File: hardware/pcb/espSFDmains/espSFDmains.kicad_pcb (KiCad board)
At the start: 2 copper layers, 59.1 x 88.9 mm, 22 parts, among them J1 Conn_01x06_Socket, J2 Conn_02x10_Odd_Even, J3 Mains, J4 Mains Motor, U1 WeMos_D1_mini_esp32, U2 TSR_1-2450, U3 SFH617A-1

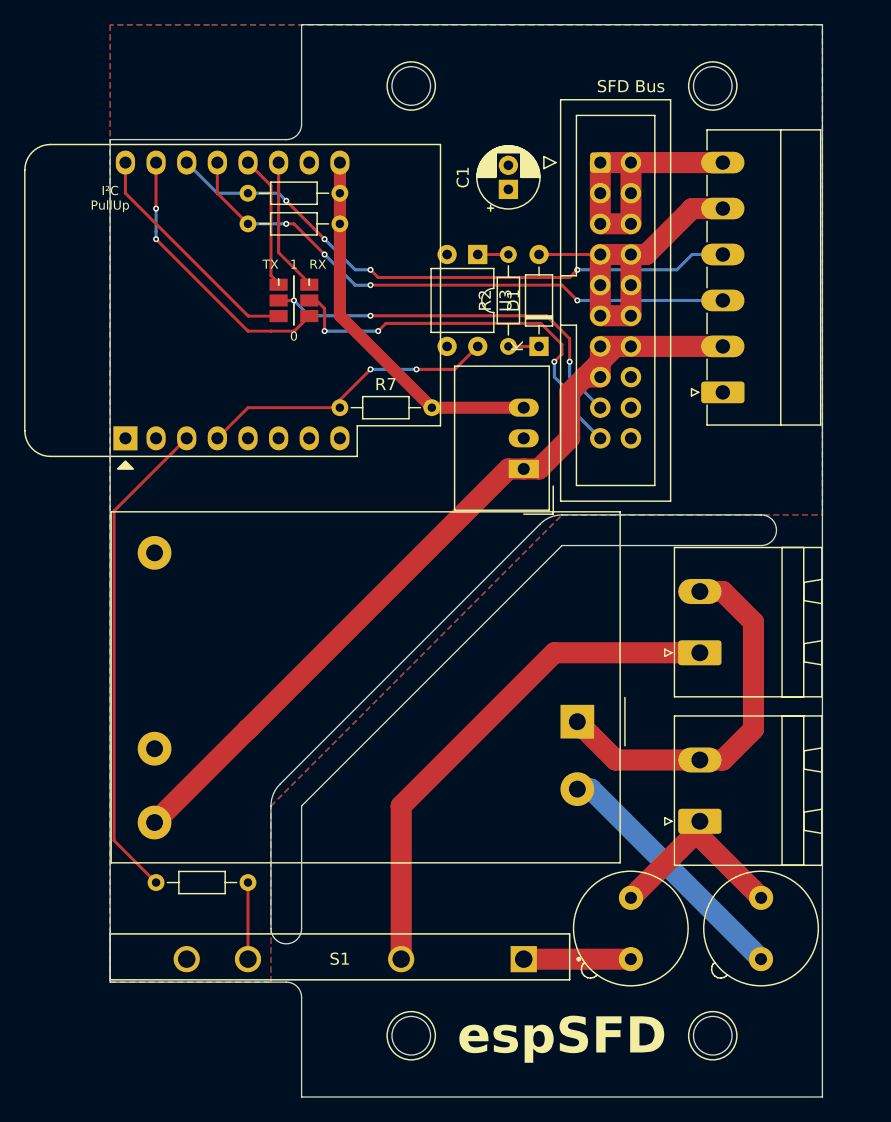
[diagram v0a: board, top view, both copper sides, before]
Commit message: bsfnbdfnb
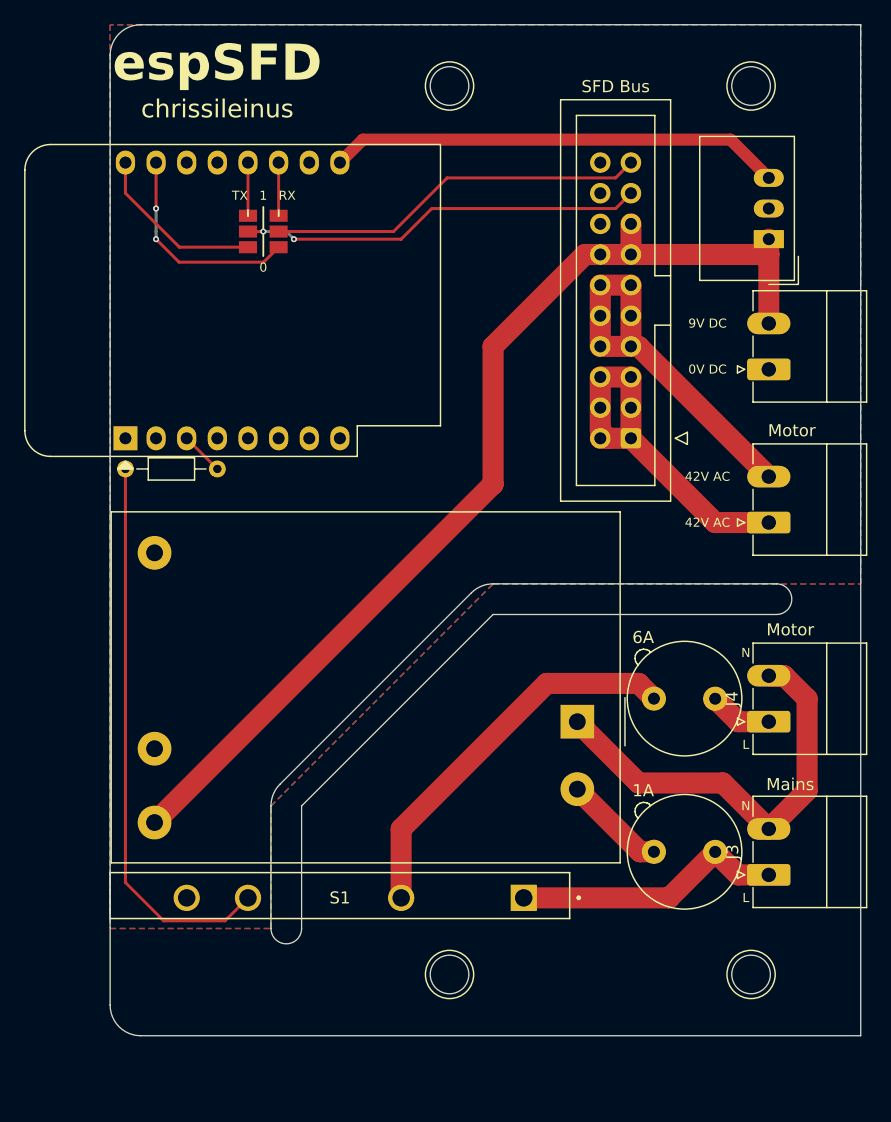
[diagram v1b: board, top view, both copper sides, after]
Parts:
- removed C1: 100µ/25V, Capacitor_THT:CP_Radial_D5.0mm_P2.00mm
- removed D1: 1N4148, Diode_THT:D_DO-35_SOD27_P7.62mm_Horizontal
- removed R2, R7: 180R, Resistor_THT:R_Axial_DIN0204_L3.6mm_D1.6mm_P7.62mm_Horizontal
- removed R5, R6: 4K7, Resistor_THT:R_Axial_DIN0204_L3.6mm_D1.6mm_P7.62mm_Horizontal
- removed U3: SFH617A-1, Package_DIP:DIP-4_W7.62mm
- added J5: Motor, Connector_Phoenix_MC:PhoenixContact_MC_1,5_2-G-3.81_1x02_P3.81mm_Horizontal, F.Cu at (143.2, 111.4)
- J1: value Conn_01x06_Socket -> VDD; footprint Connector_Phoenix_MC:PhoenixContact_MC_1,5_6-G-3.81_1x06_P3.81mm_Horizontal -> Connector_Phoenix_MC:PhoenixContact_MC_1,5_2-G-3.81_1x02_P3.81mm_Horizontal
- J3, J4: footprint Connector_Phoenix_MSTB:PhoenixContact_MSTBA_2,5_2-G-5,08_1x02_P5.08mm_Horizontal -> Connector_Phoenix_MC:PhoenixContact_MC_1,5_2-G-3.81_1x02_P3.81mm_Horizontal
- R1: value 180R -> 100R
- moved R1 34.7 mm to (97.5, 107.0), turned to 180 degrees
- moved U2 27.9 mm to (143.2, 87.9)
- moved J2 23.0 mm to (131.8, 104.5), turned to 180 degrees
- moved F2 17.9 mm to (138.7, 126.0), turned to 180 degrees
- moved J4 8.08 mm to (143.2, 127.9)
- moved J3 7.24 mm to (143.2, 140.6)
- moved JP1 6.25 mm to (102.5, 87.3)
- moved JP2 6.25 mm to (100.0, 87.3)
- moved DRA2 5.99 mm to (129.2, 148.9)
- moved F1 5.39 mm to (138.7, 138.7), turned to 180 degrees
- moved S1 5.08 mm to (107.6, 142.4)
- moved J1 4.26 mm to (143.2, 98.7)
- moved DRA1 3.17 mm to (129.2, 75.2)
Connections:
- net Net-(U1-D0) renamed En Motor
- F2 pad 1: LINE -> 230V Motor
- F2 pad 2: Net-(S1-AC_LOAD1) -> Net-(S1-AC_LOAD2)
- S1 pad 1: Net-(S1-AC_LOAD1) -> LINE
- S1 pad 2: 230V Motor -> Net-(S1-AC_LOAD2)
- U1 pad 13: SDA -> unconnected-(U1-SDA/D2-Pad13)
- U1 pad 14: SCL -> unconnected-(U1-SCL/D1-Pad14)
- U1 pad 4: Det. Motor Supply -> unconnected-(U1-SCK/D5-Pad4)
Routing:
- net SCL: track 49.2 -> 0.00 mm, vias 4 -> 0
- net SDA: track 48.1 -> 0.00 mm, vias 4 -> 0
- net Net-(S1-+LED): track 6.35 -> 46.6 mm
- net 230V Motor: track 42.7 -> 5.23 mm
- net En Motor: track 40.8 -> 3.59 mm
- net Net-(S1-AC_LOAD2): track 0.00 -> 32.2 mm
- net Det. Motor Supply: track 25.1 -> 0.00 mm, vias 2 -> 0
- net VDD: track 70.8 -> 86.7 mm
- net Net-(PS2-AC/L): track 21.1 -> 8.50 mm
- net Net-(S1-AC_LOAD1): track 8.88 -> 0.00 mm
- net Motor N: track 22.9 -> 29.8 mm
- net RX1: track 11.1 -> 4.41 mm
- net TX1: track 11.1 -> 4.41 mm
- net VCC: track 31.1 -> 37.7 mm
- net LINE: track 17.2 -> 22.7 mm
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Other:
- board size 59.1 x 88.9 mm -> 62.2 x 83.8 mm
- board text added: "1A"
- board text added: "6A"
- board text added: "9V DC"
- board text added: "Mains"
- board text added: "chrissileinus"
- board text removed: "6V DC"
- board text removed: "I²C Bus"
- board text removed: "I²C PullUp"
- board text removed: "Mains In"
- board text removed: "SCL"
- board text removed: "SDL"
